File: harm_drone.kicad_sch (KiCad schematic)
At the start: 4 parts, among them IC1 Microcontroller, J1 SYS_DEBUG

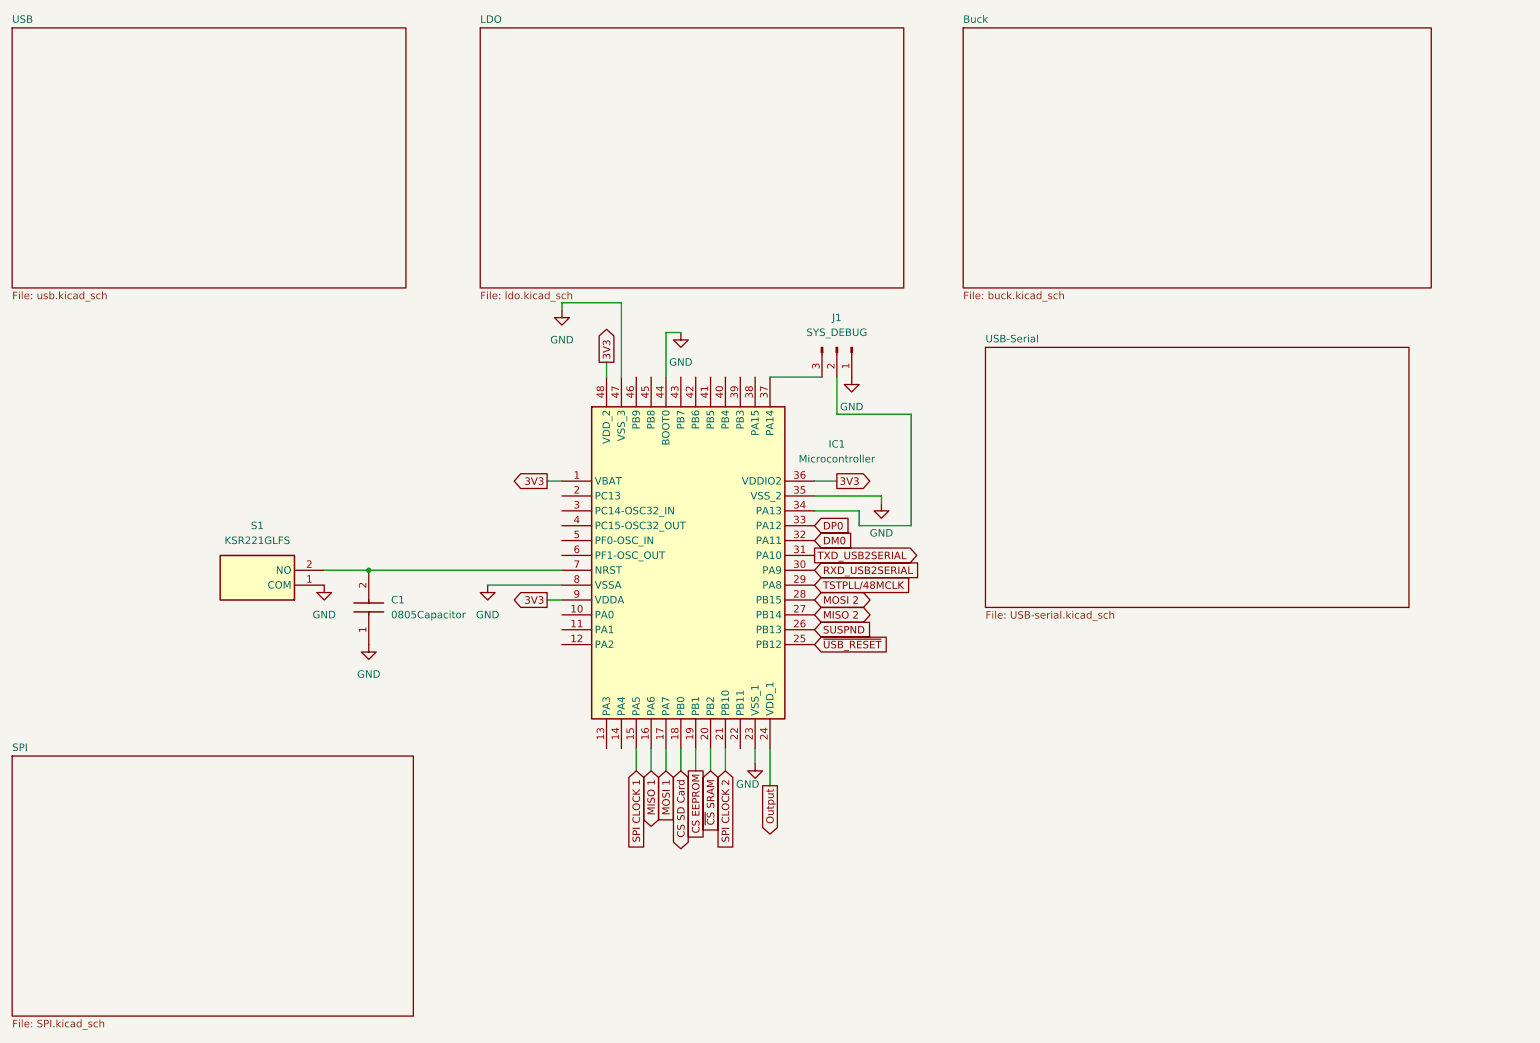
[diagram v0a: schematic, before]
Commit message: initial PCB draft!
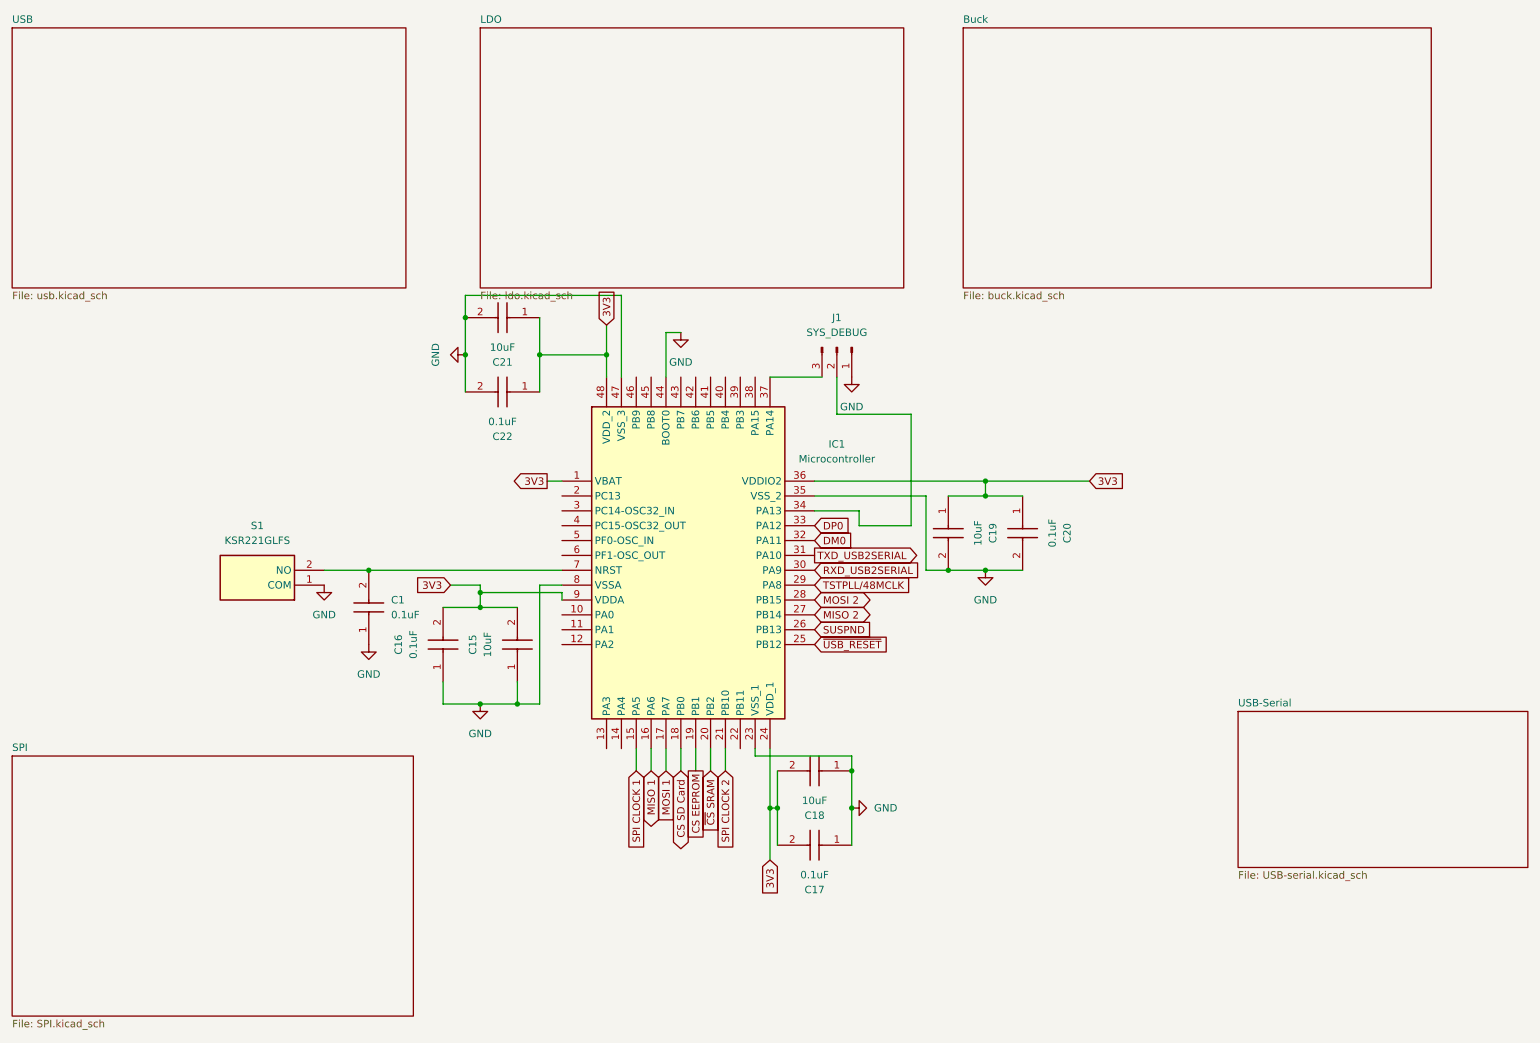
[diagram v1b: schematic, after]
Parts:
- added C15, C18, C19, C21: 10uF, Capacitor_SMD:C_0805_2012Metric, symbol group127:0805Capacitor
- added C16, C17, C20, C22: 0.1uF, Capacitor_SMD:C_0805_2012Metric, symbol group127:0805Capacitor
- C1: value 0805Capacitor -> 0.1uF
- IC1: footprint (none) -> group127:Microcontroller
- J1: footprint Connector_PinHeader_2.54mm:PinHeader_1x02_P2.54mm_Vertical -> Connector_PinHeader_2.54mm:PinHeader_1x03_P2.54mm_Vertical
- S1: footprint (none) -> group127:Button
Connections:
- net Output is gone; now on net 3V3: IC1.24 (VDD_1)
- net 3V3: now also C15.2, C16.2, C17.2, C18.2, C19.1, C20.1, C21.1, C22.1
- net GND: now also C15.1, C16.1, C17.1, C18.1, C19.2, C20.2, C21.2, C22.2

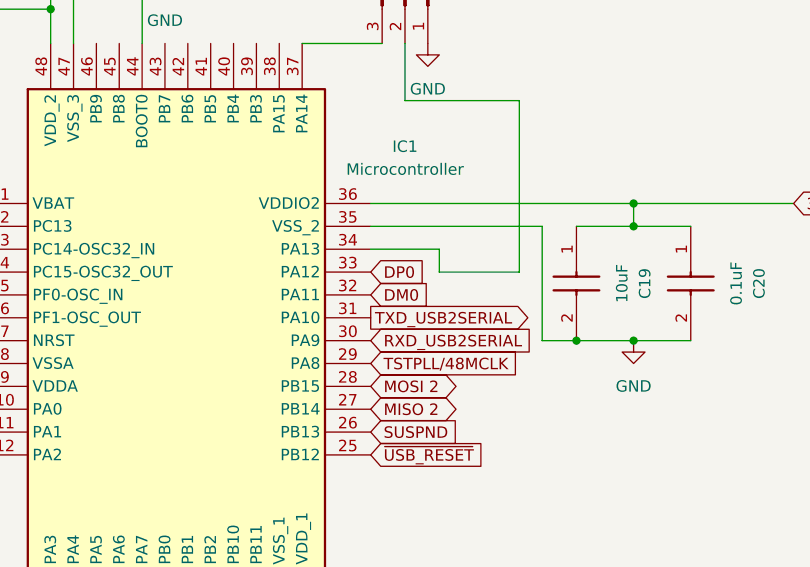
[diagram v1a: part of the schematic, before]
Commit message: namespace change
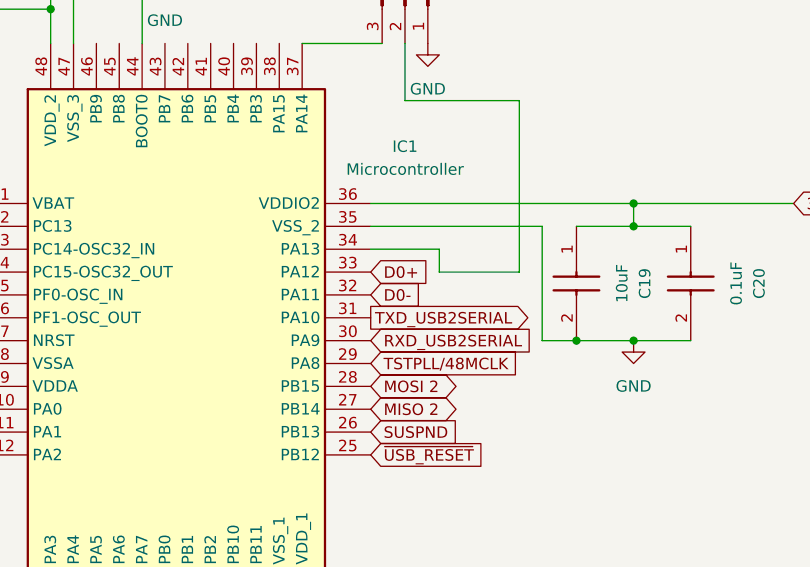
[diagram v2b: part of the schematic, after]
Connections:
- net DM0 renamed D0-
- net DP0 renamed D0+
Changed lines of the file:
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@@
 		)
 	)
-	(global_label "DM0"
+	(global_label "D0-"
 		(shape input)
 		(at 161.29 107.95 0)
@@
 		)
 	)
-	(global_label "DP0"
+	(global_label "D0+"
 		(shape input)
 		(at 161.29 105.41 0)
